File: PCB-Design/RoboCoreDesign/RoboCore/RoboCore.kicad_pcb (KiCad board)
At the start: 4 copper layers, 68 x 60 mm, 81 parts, among them IC1 DRV8245SQRXZRQ1, IC2 DRV8245SQRXZRQ1, J1 SS-52400-002, J2 B2B-PH-SM4-TB, Q1 BC817, Q2 BC817, U1 MCP73871, U2 CP2102N-Axx-xQFN20, U3 USBLC6-2SC6, U4 ESP32-C3-WROOM-02-H4, U5 MPU-6050

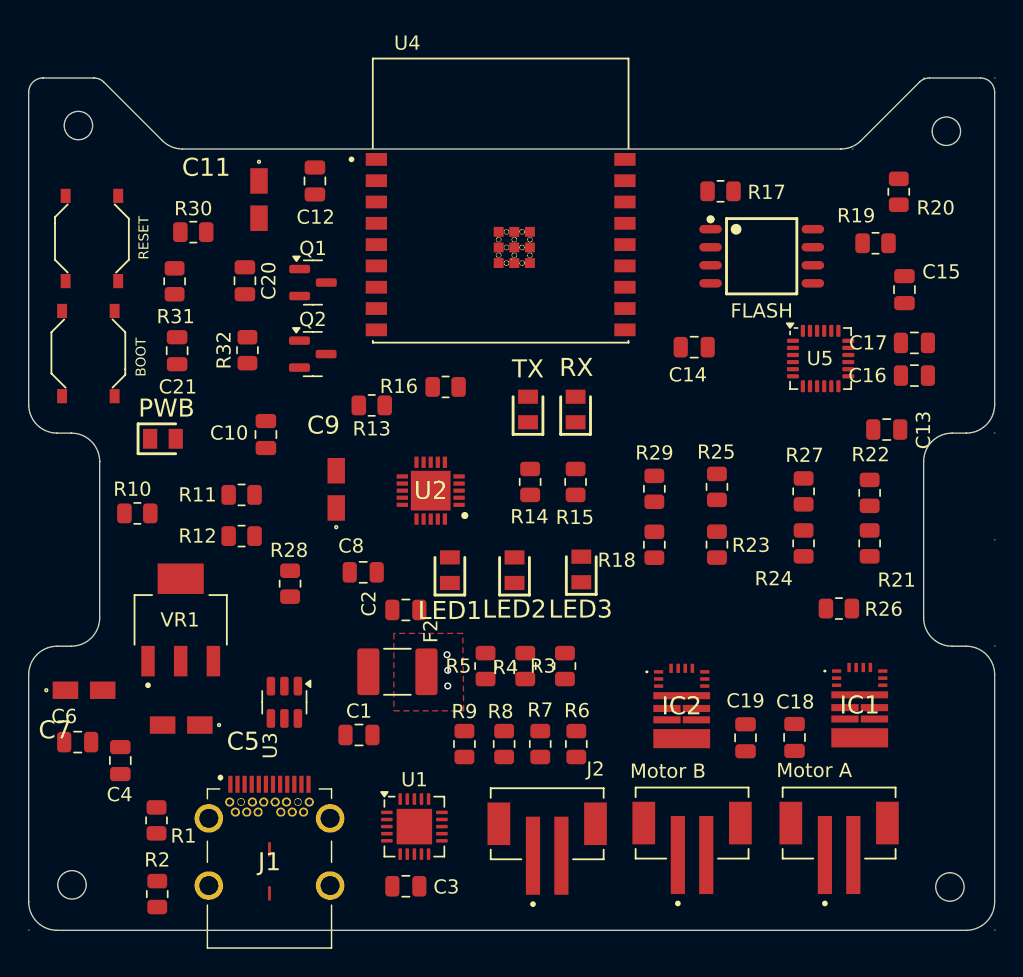
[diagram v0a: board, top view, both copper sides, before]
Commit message: made improvements to the PCB
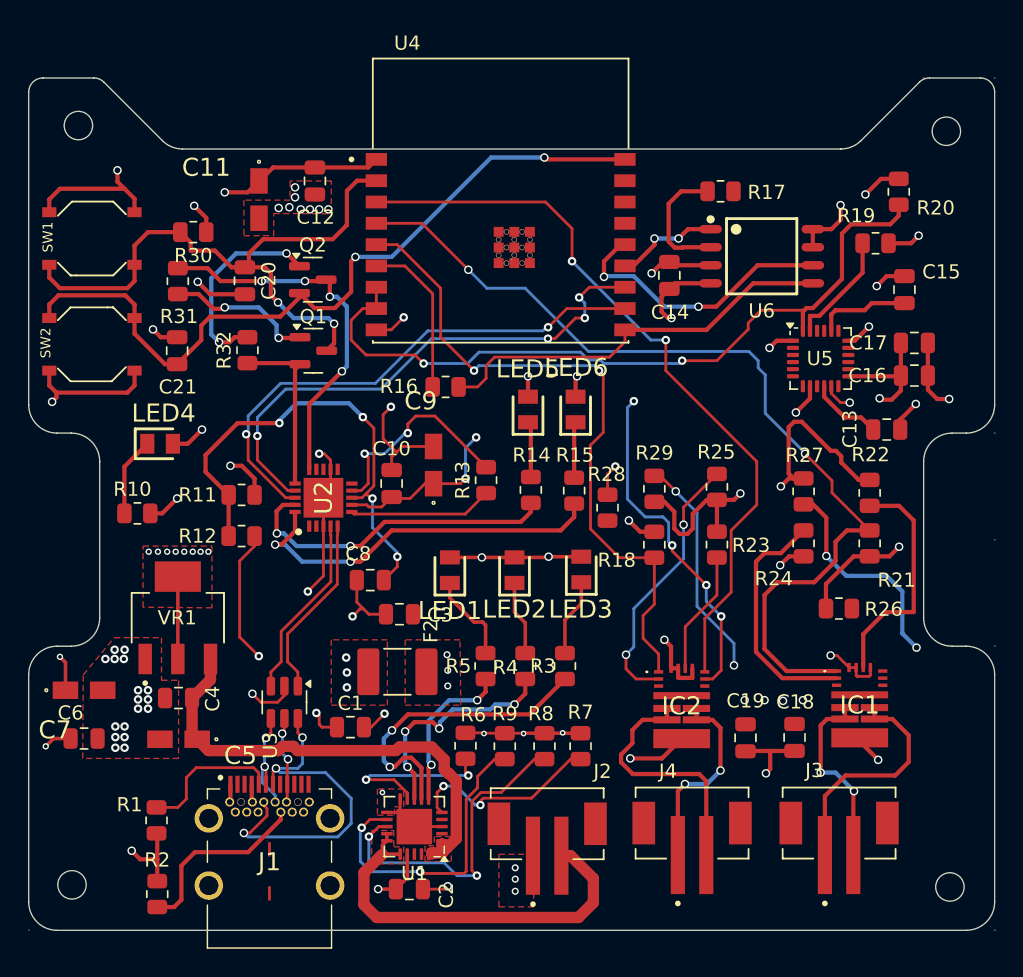
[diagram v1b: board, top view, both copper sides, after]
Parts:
- J3: renamed from Motor A
- J4: renamed from Motor B
- moved R28 23.0 mm to (171.8, 109.1)
- moved C2 19.7 mm to (157.8, 135.9), turned to 0 degrees
- moved C3 19.2 mm to (157.1, 116.6)
- moved R13 9.62 mm to (163.2, 107.2), turned to 90 degrees
- moved C10 9.50 mm to (156.6, 107.4)
- moved R6 7.80 mm to (161.8, 125.9)
- moved U2 7.57 mm to (151.8, 108.4), turned to 90 degrees
- moved C9 7.06 mm to (159.5, 106.1)
- moved C4 6.01 mm to (141.6, 122.5), turned to 180 degrees
- moved C14 5.34 mm to (176.1, 92.8), turned to 90 degrees
- moved Q2 5.24 mm to (151.0, 93.0)
- moved Q1 4.80 mm to (151.0, 98.0)
- moved R7 2.84 mm to (169.8, 125.9)
- moved R8 2.84 mm to (167.3, 125.9)
- moved R9 2.84 mm to (164.5, 125.9)
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- renumbered PWB to LED4, TX to LED5, RX to LED6, RESET to SW1, BOOT to SW2, FLASH to U6
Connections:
- net Net-(R3--) renamed /CHARGING_POWER_GOOD
- net Net-(R4--) renamed /CHARGED
- net Net-(R5--) renamed /CHARGING
- U1 pad 14: Net-(U1-V_{BAT_SENSE}) -> /VBAT
- U1 pad 15: Net-(U1-V_{BAT_SENSE}) -> /VBAT
- U1 pad 16: Net-(U1-V_{BAT_SENSE}) -> /VBAT
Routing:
- net GND: track 0.00 -> 153.7 mm, vias 0 -> 62
- net +3.3V: track 0.00 -> 79.5 mm, vias 0 -> 26
- net /ESP32_BOARD_CONNECTION/nFAULT_A: track 0.00 -> 65.7 mm, vias 0 -> 2
- net /ESP32_BOARD_CONNECTION/BOOT: track 0.00 -> 53.9 mm, vias 0 -> 2
- net /ESP32_BOARD_CONNECTION/I2C_SDA: track 0.00 -> 53.6 mm, vias 0 -> 2
- net /ESP32_BOARD_CONNECTION/DIR_B: track 0.00 -> 53.3 mm, vias 0 -> 2
- net /ESP32_BOARD_CONNECTION/nFAULT_B: track 0.00 -> 47.5 mm, vias 0 -> 2
- net /ESP32_BOARD_CONNECTION/EN: track 0.00 -> 44.1 mm, vias 0 -> 2
- net /ESP32_BOARD_CONNECTION/RX_TX: track 0.00 -> 37.6 mm, vias 0 -> 4
- net /ESP32_BOARD_CONNECTION/TX_RX: track 0.00 -> 37.3 mm, vias 0 -> 2
- net Net-(C8--): track 0.00 -> 34.0 mm, vias 0 -> 4
- net +5V: track 0.00 -> 33.6 mm
- net /ESP32_BOARD_CONNECTION/SPI_MOSI: track 0.00 -> 29.0 mm
- net /VBAT: track 0.00 -> 28.5 mm
- net Net-(R15--): track 0.00 -> 26.9 mm, vias 0 -> 2
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- added copper zone on F.Cu, net +3.3V
- added copper zone on F.Cu, net +5V
- added copper zone on F.Cu, net /VBAT
- added copper zone on F.Cu, net /VBUS
- added copper zone on F.Cu, net GND
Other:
- outline, holes or cut-outs redrawn
